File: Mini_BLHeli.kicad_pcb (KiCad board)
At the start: 2 copper layers, 28.5 x 27.6 mm, 56 parts, among them J1 Conn_01x06, Q1 HY12P03, Q2 HY1503C1, Q3 Q_NMOS_GSD, Q4 HY12P03, Q5 HY1503C1, Q6 Q_NMOS_GSD, Q7 HY12P03, Q8 HY1503C1, Q9 Q_NMOS_GSD, U1 EFM8BB21F16G-C-QFN20, U2 TLV70033_SOT23-5

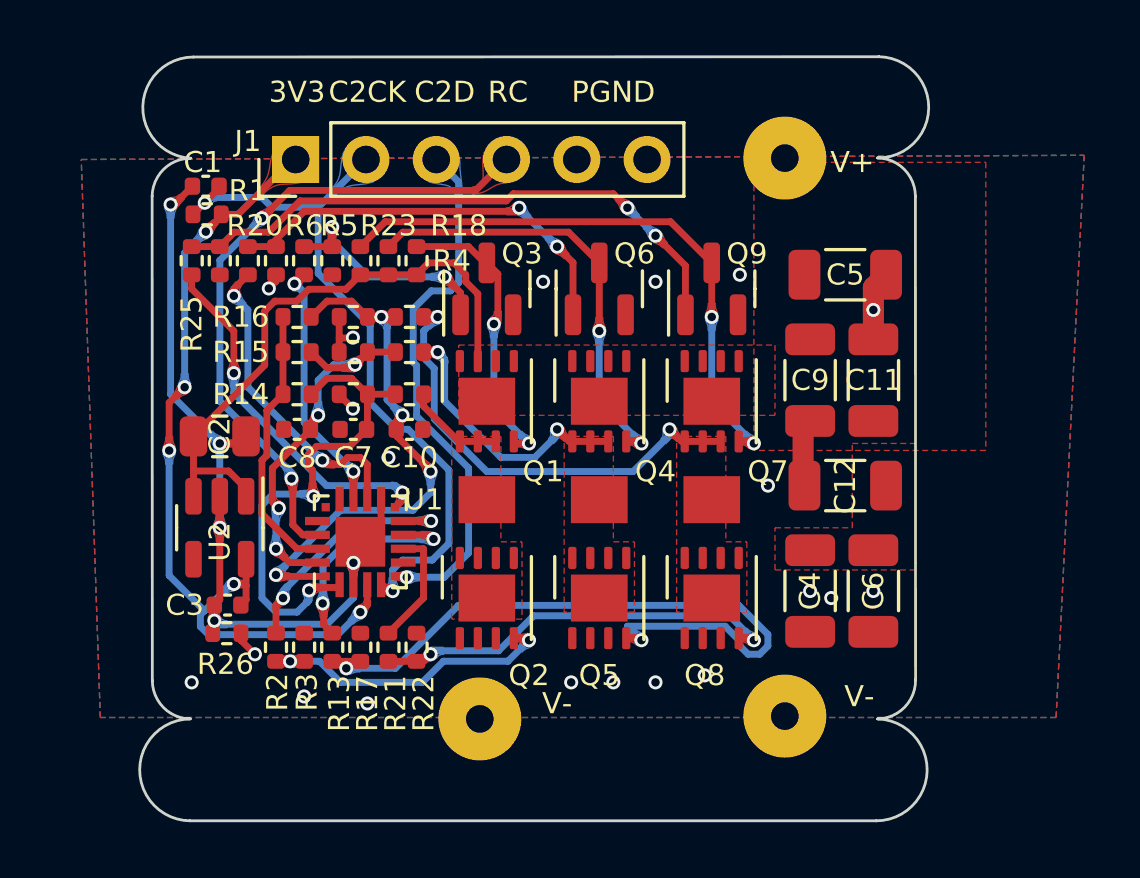
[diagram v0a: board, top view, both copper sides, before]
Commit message: update for new version
Signed-off-by: huangzzk <huangcmzzk@gmail.com>
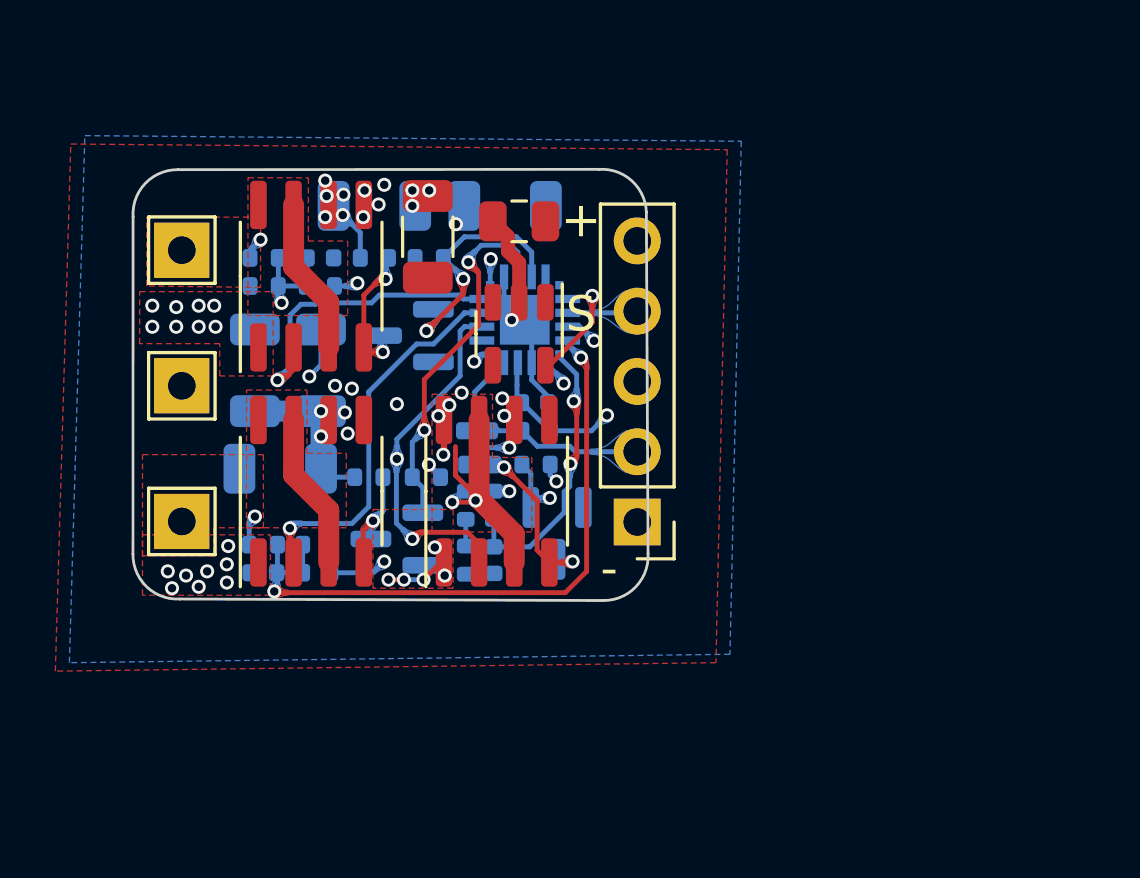
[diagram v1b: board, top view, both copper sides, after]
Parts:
- removed A, B, C, V+, V- (x2): , 
- removed Q7: HY12P03, Package_DFN_QFN:DFN-8-1EP_3x3mm_P0.65mm_EP1.7x2.05mm
- removed Q8: HY1503C1, Package_DFN_QFN:DFN-8-1EP_3x3mm_P0.65mm_EP1.7x2.05mm
- removed Q9: Q_NMOS_GSD, Package_TO_SOT_SMD:SOT-23
- removed R17, R18, R19, R22, R23, R24: 10K, Resistor_SMD:R_0402_1005Metric
- removed R20, R21, R25: 20R, Resistor_SMD:R_0402_1005Metric
- removed R26: 0R, Resistor_SMD:R_0402_1005Metric
- added TP1: TestPoint, TestPoint:TestPoint_THTPad_2.0x2.0mm_Drill1.0mm, F.Cu at (123.6, 92.6)
- added TP2: TestPoint, TestPoint:TestPoint_THTPad_2.0x2.0mm_Drill1.0mm, F.Cu at (123.6, 102.4)
- added TP3: TestPoint, TestPoint:TestPoint_THTPad_2.0x2.0mm_Drill1.0mm, F.Cu at (123.6, 97.5)
- C1, C10, C11, C3, C4, C5, C6, C7, C8, C9, Q6, R1, R10, R11, R12, R14, R15, R16, R3, R4, R5, R7, R8, R9, U1: moved to B.Cu
- J1: value Conn_01x06 -> Conn_01x05; footprint Connector_PinHeader_2.54mm:PinHeader_1x06_P2.54mm_Vertical -> Connector_PinHeader_2.54mm:PinHeader_1x05_P2.54mm_Vertical
- Q1: value HY12P03 -> HYG170C03LR1S; footprint Package_DFN_QFN:DFN-8-1EP_3x3mm_P0.65mm_EP1.7x2.05mm -> Package_SO:SO-8_3.9x4.9mm_P1.27mm
- Q2: value HY1503C1 -> HYG170C03LR1S; footprint Package_DFN_QFN:DFN-8-1EP_3x3mm_P0.65mm_EP1.7x2.05mm -> Package_SO:SO-8_3.9x4.9mm_P1.27mm
- Q3: value Q_NMOS_GSD -> HYG170C03LR1S; footprint Package_TO_SOT_SMD:SOT-23 -> Package_SO:SO-8_3.9x4.9mm_P1.27mm
- Q4: value HY12P03 -> Q_NMOS_GSD; footprint Package_DFN_QFN:DFN-8-1EP_3x3mm_P0.65mm_EP1.7x2.05mm -> Package_TO_SOT_SMD:SOT-23; moved to B.Cu
- Q5: value HY1503C1 -> Q_NMOS_GSD; footprint Package_DFN_QFN:DFN-8-1EP_3x3mm_P0.65mm_EP1.7x2.05mm -> Package_TO_SOT_SMD:SOT-23; moved to B.Cu
- R13, R2, R6: value 20R -> 10K; moved to B.Cu
- moved C4 21.6 mm to (126.2, 96.9), turned to 90 degrees
- moved C6 21.5 mm to (128.6, 96.9), turned to 90 degrees
- moved C11 19.4 mm to (127.2, 100.5), turned to 180 degrees
- moved J1 18.0 mm to (140.1, 102.4), turned to 180 degrees
- moved C12 17.6 mm to (132.5, 92.1), turned to 90 degrees
- moved C5 17.2 mm to (130.6, 91.0)
- moved C9 14.7 mm to (135.3, 91.0), turned to 0 degrees
- moved R2 14.5 mm to (130.6, 92.9), turned to 0 degrees
- moved R1 14.2 mm to (136.4, 99.1)
- moved C2 13.3 mm to (135.8, 91.5), turned to 180 degrees
- moved C3 13.3 mm to (136.3, 98.1), turned to 0 degrees
- moved C1 13.2 mm to (134.3, 99.1)
- moved U2 12.9 mm to (135.8, 95.6)
- moved U1 9.99 mm to (136.0, 95.1)
- moved R13 9.89 mm to (136.4, 100.3), turned to 180 degrees
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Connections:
- C10 pad 2: /PGND -> GND
- C11 pad 2: /PGND -> GND
- C12 pad 2: /PGND -> GND
- C4 pad 2: /PGND -> GND
- C5 pad 2: /PGND -> GND
- C6 pad 2: /PGND -> GND
- C7 pad 2: /PGND -> GND
- C8 pad 2: /PGND -> GND
- C9 pad 2: /PGND -> GND
- J1 pad 1: +3V3 -> GND
- J1 pad 5: /PGND -> +BATT
- Q1 pad 1: /HBridge/A -> GND
- Q1 pad 2: /HBridge/A -> /AL
- Q1 pad 7: +BATT -> /HBridge/A
- Q1 pad 8: +BATT -> /HBridge/A
- Q2 pad 1: /PGND -> GND
- Q2 pad 2: /PGND -> /BL
- Q2 pad 3: /PGND -> /HBridge/B
- Q2 pad 5: /HBridge/A -> +BATT
- Q2 pad 6: /HBridge/A -> +BATT
- Q2 pad 7: /HBridge/A -> /HBridge/B
- Q2 pad 8: /HBridge/A -> /HBridge/B
- Q3 pad 1: Net-(Q3-Pad1) -> GND
- Q3 pad 2: /PGND -> /CL
- Q3 pad 3: Net-(Q1-Pad4) -> /HBridge/C
- Q4 pad 1: /HBridge/B -> /AH
- Q4 pad 2: /HBridge/B -> GND
- Q4 pad 3: /HBridge/B -> Net-(Q1-Pad4)
- Q5 pad 1: /PGND -> /BH
- Q5 pad 2: /PGND -> GND
- Q5 pad 3: /PGND -> Net-(Q2-Pad4)
- Q6 pad 1: Net-(Q6-Pad1) -> /CH
- Q6 pad 2: /PGND -> GND
- Q6 pad 3: Net-(Q4-Pad4) -> Net-(Q3-Pad4)
- R10 pad 2: /PGND -> GND
- R11 pad 2: /PGND -> GND
- R12 pad 2: /PGND -> GND
- R13 pad 1: /BL -> GND
- R13 pad 2: Net-(Q5-Pad4) -> /CH
- R2 pad 1: /AL -> +BATT
- R2 pad 2: Net-(Q2-Pad4) -> Net-(Q1-Pad4)
- R3 pad 1: /PGND -> +BATT
- R4 pad 1: Net-(Q1-Pad4) -> +BATT
- R4 pad 2: +BATT -> Net-(Q3-Pad4)
- R5 pad 1: /PGND -> GND
- R5 pad 2: Net-(Q3-Pad1) -> /AH
- R6 pad 1: Net-(Q3-Pad1) -> GND
- R6 pad 2: /AH -> /BH
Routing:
- net Net-(Q5-Pad4): track 25.3 -> 0.00 mm, vias 2 -> 0
- net Net-(Q9-Pad1): track 21.5 -> 0.00 mm, vias 2 -> 0
- net Net-(Q7-Pad4): track 21.4 -> 0.00 mm, vias 2 -> 0
- net /RC: track 23.6 -> 2.54 mm, vias 2 -> 0
- net /CC: track 9.96 -> 28.8 mm, vias 0 -> 4
- net +3V3: track 30.8 -> 13.3 mm, vias 5 -> 2
- net /C2CK: track 26.3 -> 8.94 mm, vias 2 -> 0
- net Net-(Q4-Pad4): track 16.0 -> 0.00 mm, vias 2 -> 0
- net Net-(Q6-Pad1): track 15.3 -> 0.00 mm, vias 2 -> 0
- net Net-(Q8-Pad4): track 14.8 -> 0.00 mm, vias 2 -> 0
- net /C2D: track 19.5 -> 7.26 mm
- net /VB: track 13.7 -> 23.9 mm, vias 4 -> 2
- net /PGND: track 9.05 -> 0.00 mm, vias 20 -> 0
- net /CL: track 4.31 -> 12.9 mm, vias 0 -> 2
- net +BATT: track 21.7 -> 13.2 mm, vias 0 -> 19
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- added copper zone on In2.Cu, net +BATT
- added copper zone on In1.Cu, net /HBridge/C
- added copper zone on B.Cu, net GND
- added copper zone on F.Cu, net GND
- added copper zone on In1.Cu, net GND
- added copper zone on In2.Cu, net GND
- removed copper zone on B.Cu, net /PGND
- removed copper zone on F.Cu, net /PGND
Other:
- board size 28.5 x 27.6 mm -> 18.6 x 15.6 mm
- copper layers 2 -> 4
- board text added: "+"
- board text added: "-"
- board text added: "S"
- board text removed: "3V3"
- board text removed: "C2CK"
- board text removed: "C2D"
- board text removed: "PGND"
- board text removed: "RC"
